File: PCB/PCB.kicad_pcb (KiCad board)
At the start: 2 copper layers, 115 x 77 mm, 153 parts, among them J1 Conn_01x06, J2 Screw_Terminal_01x04, J3 Screw_Terminal_01x08, J4 Conn_02x06_Odd_Even, J5 Conn_01x03, U1 ESP32-S3, U10 TPS22918DBV, U2 PC817, U3 PC817, U4 ADuM1411, U5 ATM90E36A-AU-R, U6 HLK-5M05, U7 B0303S-1WR3, U8 BQ24073RGT, U9 TLV75733PDRV, Y1 ABM8W-16.3840MHZ-4-B1U-T3

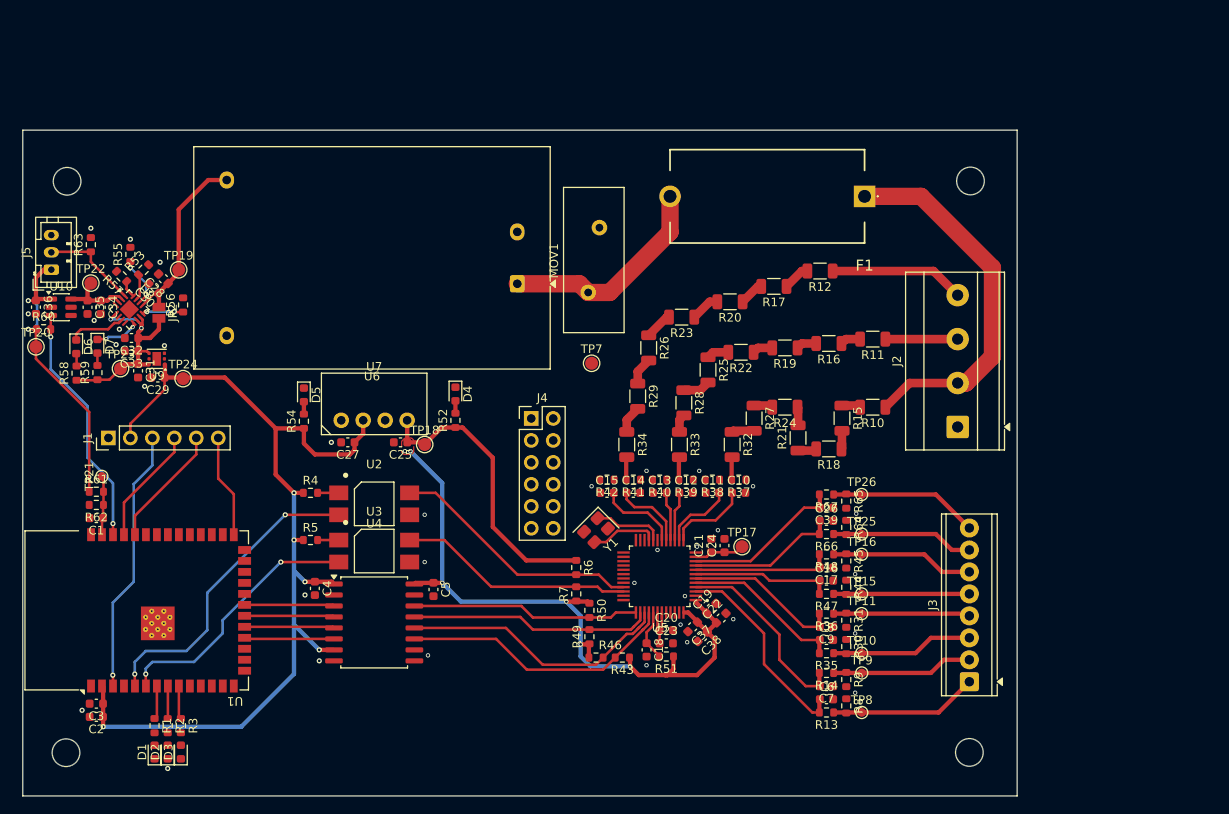
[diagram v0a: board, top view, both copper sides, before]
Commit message: edited the PCB layout
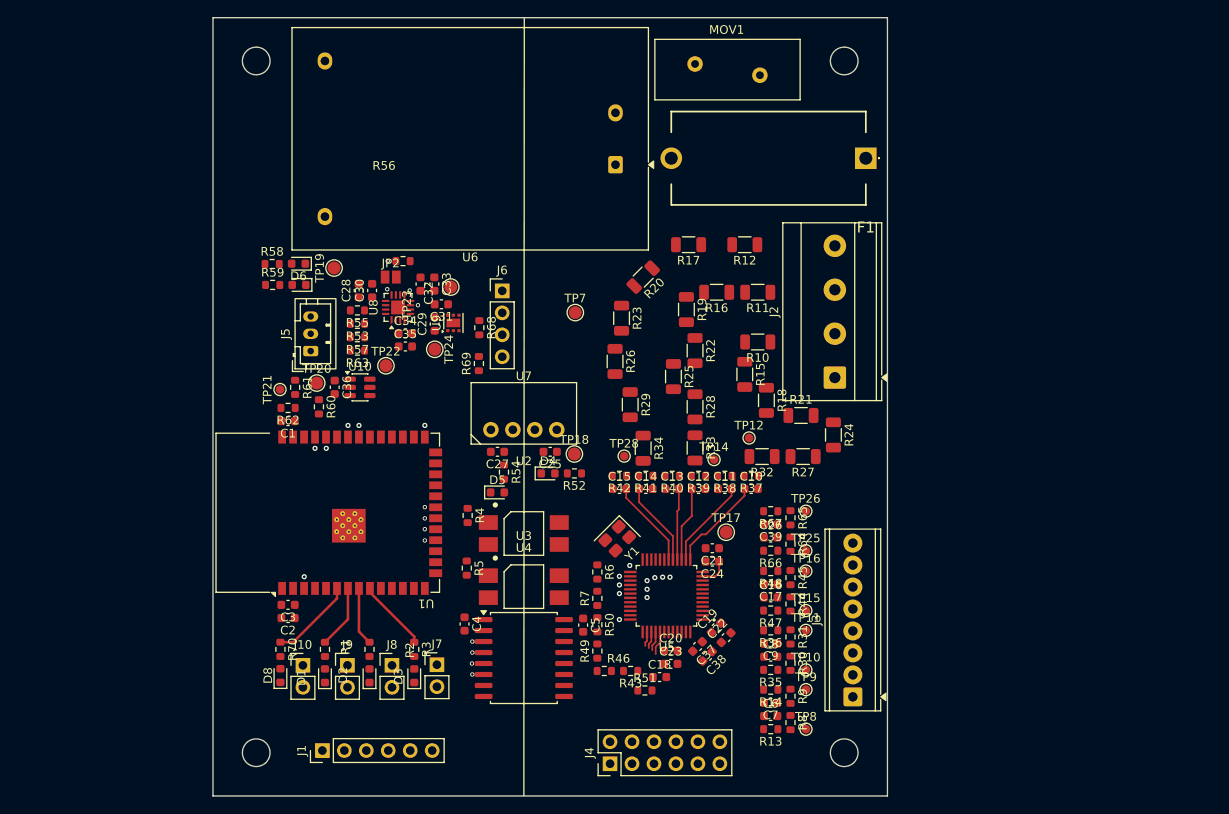
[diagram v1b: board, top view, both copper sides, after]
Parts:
- added D8: LED_L3, LED_SMD:LED_0603_1608Metric, F.Cu at (89.8, 126.1)
- added J10: Conn_01x02, Connector_PinHeader_2.54mm:PinHeader_1x02_P2.54mm_Vertical, F.Cu at (92.4, 124.9)
- added J6: Conn_01x04, Connector_PinHeader_2.54mm:PinHeader_1x04_P2.54mm_Vertical, F.Cu at (115.5, 81.6)
- added J7: Conn_01x02, Connector_PinHeader_2.54mm:PinHeader_1x02_P2.54mm_Vertical, F.Cu at (107.9, 124.8)
- added J8: Conn_01x02, Connector_PinHeader_2.54mm:PinHeader_1x02_P2.54mm_Vertical, F.Cu at (102.7, 124.9)
- added J9: Conn_01x02, Connector_PinHeader_2.54mm:PinHeader_1x02_P2.54mm_Vertical, F.Cu at (97.5, 124.9)
- added R68: 10k, Resistor_SMD:R_0603_1608Metric, F.Cu at (112.8, 85.8)
- added R69: 10k, Resistor_SMD:R_0603_1608Metric, F.Cu at (112.8, 90.0)
- added R70: 1k, Resistor_SMD:R_0603_1608Metric, F.Cu at (89.8, 123.0)
- added TP12: TestPoint, TestPoint:TestPoint_Pad_D1.0mm, F.Cu at (144.0, 98.6)
- added TP14: TestPoint, TestPoint:TestPoint_Pad_D1.0mm, F.Cu at (139.9, 101.1)
- added TP28: TestPoint, TestPoint:TestPoint_Pad_D1.0mm, F.Cu at (129.6, 100.7)
- moved J1 43.8 mm to (94.7, 134.8)
- moved J4 41.0 mm to (127.9, 136.3), turned to 90 degrees
- moved TP23 39.3 mm to (109.5, 81.2), turned to -90 degrees
- moved C35 37.0 mm to (104.3, 88.0), turned to 0 degrees
- moved C31 35.9 mm to (108.4, 83.1), turned to 180 degrees
- moved C33 35.9 mm to (107.6, 80.8), turned to -90 degrees
- moved U10 35.8 mm to (99.0, 92.8)
- moved C36 35.8 mm to (96.1, 92.7)
- moved TP22 35.4 mm to (102.0, 90.2)
- moved C34 35.4 mm to (104.3, 86.5), turned to 0 degrees
- moved U9 34.6 mm to (109.8, 85.3), turned to 90 degrees
- moved C32 34.0 mm to (106.0, 80.8), turned to -90 degrees
- moved R63 33.2 mm to (98.7, 88.5), turned to 180 degrees
- moved R60 33.1 mm to (94.2, 95.0), turned to -90 degrees
- moved TP20 32.7 mm to (94.0, 92.2)
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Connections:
- net /Digital/EN renamed /EN
- net /Digital/IO0 renamed /IO0
- net /Digital/IO14 renamed /IO14
- net /Digital/IO17 renamed /IO17
- net /Digital/IO18 renamed /IO18
- net /Digital/IO21 renamed /IO21
- net /Digital/IO3 renamed /IO3
- net /Digital/IO35 renamed /IO35
- net /Digital/IO36 renamed /IO36
- net /Digital/IO37 renamed /IO37
- net /Digital/IO38 renamed /IO38
- net /Digital/IO39 renamed /IO39
- net /Digital/IO4 renamed /IO4
- net /Digital/IO42 renamed /IO42
- net /Digital/IO46 renamed /IO46
- net /Digital/IO47 renamed /IO47
- net /Digital/IO8 renamed /IO8
- net /Digital/IO9 renamed /IO9
- net /Digital/LED_L1 renamed /LED_L1
- net /Digital/LED_L2 renamed /LED_L2
- net /Digital/LED_L3 renamed /LED_L3
- net /Digital/MCU_CS renamed /MCU_CS
- net /Digital/MCU_MISO renamed /MCU_MISO
- net /Digital/MCU_MOSI renamed /MCU_MOSI
- net /Digital/MCU_SCLK renamed /MCU_SCLK
- net /Digital/RXD0 renamed /RXD0
- net /Digital/TXD0 renamed /TXD0
- net /Digital/USB_D+ renamed /USB_D+
- net /Digital/USB_D- renamed /USB_D-
- net /Energy Metering/I1N renamed /I1N
- net /Energy Metering/I1P renamed /I1P
- net /Energy Metering/I2N renamed /I2N
- net /Energy Metering/I2P renamed /I2P
- net /Energy Metering/I3N renamed /I3N
- net /Energy Metering/I3P renamed /I3P
- net /Energy Metering/I4N renamed /I4N
- net /Energy Metering/I4P renamed /I4P
- net /Energy Metering/OSCI renamed /OSCI
- net /Energy Metering/OSCO renamed /OSCO
- net /Energy Metering/V1N renamed /V1N
- net /Energy Metering/V1P renamed /V1P
- net /Energy Metering/V2N renamed /V2N
- net /Energy Metering/V2P renamed /V2P
- net /Energy Metering/V3N renamed /V3N
- net /Energy Metering/V3P renamed /V3P
- net /Energy Metering/VREF renamed /VREF
- net /Supply/CHG renamed /CHG
- net /Supply/ILIM renamed /ILIM
- net /Supply/ISET renamed /ISET
- net /Supply/PG renamed /PG
- net /Supply/TD renamed /TD
- net /Supply/TMR renamed /TMR
- net /Supply/TS renamed /TS
- J4 pad 1: /Energy Metering/CF4 -> /IRQ0
- J4 pad 10: /Energy Metering/CF2 -> /ZX2
- J4 pad 12: /Energy Metering/CF3 -> /ZX0
- J4 pad 2: /Energy Metering/ZX0 -> /DMA
- J4 pad 3: /Energy Metering/WARN -> /CF2
- J4 pad 4: /Energy Metering/ZX1 -> /CF4
- J4 pad 5: /Energy Metering/IRQ0 -> /IRQ1
- J4 pad 6: /Energy Metering/ZX2 -> /CF1
- J4 pad 7: /Energy Metering/IRQ1 -> /CF3
- J4 pad 8: /Energy Metering/CF1 -> /WARN
- J4 pad 9: /Energy Metering/DMA -> /ZX1
- U1 pad 25: /Digital/IO48 -> /PMC_1
- U1 pad 26: /Digital/IO45 -> /PMC_0
- U1 pad 33: /Digital/IO40 -> /SDA
- U1 pad 34: /Digital/IO41 -> /SCL
- U1 pad 5: /Digital/PMC_0 -> /IO5
- U1 pad 6: /Digital/PMC_1 -> /LED_WIFI
- U2 pad 2: /Digital/PMC_0 -> /PMC_0
- U3 pad 2: /Digital/PMC_1 -> /PMC_1
- U5 pad 22: /Energy Metering/ZX0 -> /ZX0
- U5 pad 23: /Energy Metering/ZX1 -> /ZX1
- U5 pad 24: /Energy Metering/ZX2 -> /ZX2
- U5 pad 25: /Energy Metering/CF1 -> /CF1
- U5 pad 26: /Energy Metering/CF2 -> /CF2
- U5 pad 27: /Energy Metering/CF3 -> /CF3
- U5 pad 28: /Energy Metering/CF4 -> /CF4
- U5 pad 29: /Energy Metering/WARN -> /WARN
- U5 pad 30: /Energy Metering/IRQ0 -> /IRQ0
- U5 pad 31: /Energy Metering/IRQ1 -> /IRQ1
- U5 pad 36: /Energy Metering/DMA -> /DMA
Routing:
- net +3V3PWR: track 114.7 -> 0.00 mm, vias 6 -> 0
- net +3V3: track 112.8 -> 0.00 mm, vias 5 -> 0
- net L1: track 43.3 -> 0.00 mm
- net /Digital/PMC_0: track 36.0 -> 0.00 mm, vias 2 -> 0
- net +VBAT_IN: track 34.6 -> 0.00 mm, vias 2 -> 0
- net /EN: track 30.6 -> 0.00 mm
- net /Digital/PMC_1: track 30.3 -> 0.00 mm, vias 2 -> 0
- net MISO: track 32.3 -> 2.28 mm
- net MOSI: track 31.8 -> 1.99 mm
- net PM0: track 29.3 -> 0.00 mm
- net BAT_SW: track 28.4 -> 0.00 mm, vias 2 -> 0
- net PM1: track 27.2 -> 0.00 mm
- net +VIN: track 26.4 -> 0.00 mm, vias 2 -> 0
- net ~{CS}: track 26.4 -> 0.00 mm
- net SCLK: track 28.1 -> 1.69 mm
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- removed copper zone on F.Cu, net +3V3PWR
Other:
- board size 115 x 77 mm -> 78 x 90 mm

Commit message: PCB routing and adjusts
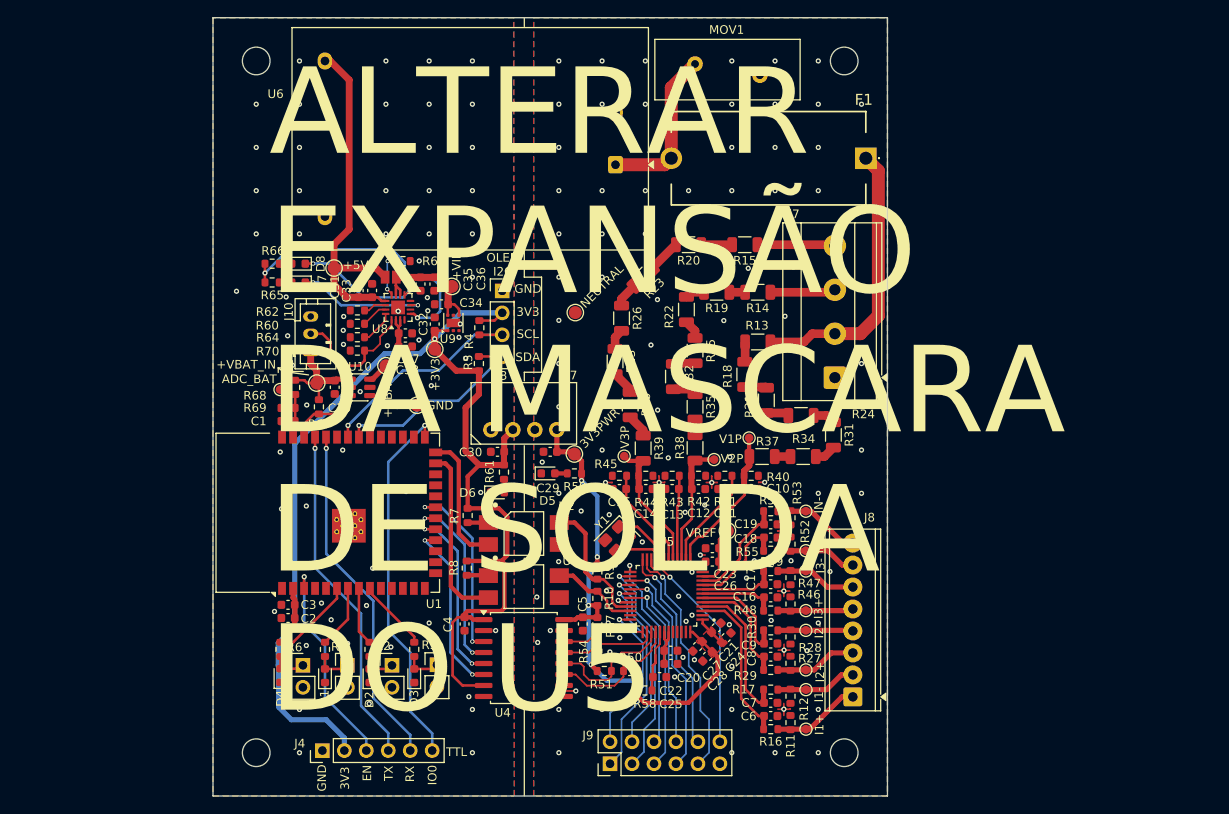
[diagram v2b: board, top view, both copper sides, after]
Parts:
- added TP21: TestPoint, TestPoint:TestPoint_Pad_D1.5mm, F.Cu at (105.6, 94.8)
- moved D8 2.45 mm to (91.9, 78.4)
- moved R66 2.45 mm to (88.8, 78.4)
- moved D7 2.17 mm to (91.9, 80.6)
- moved R65 2.13 mm to (88.8, 80.6)
- moved TP13 0.21 mm to (141.5, 109.3)
- moved TP17 0.16 mm to (109.6, 81.1)
- moved C5 0.13 mm to (124.8, 120.1)
- renumbered C26 to C18, C39 to C19, C18 to C20, C19 to C21, C20 to C22, C21 to C23, C22 to C24, C23 to C25, C24 to C26, C37 to C27, C38 to C28, C25 to C29, C27 to C30, C28 to C31, C29 to C32, C30 to C33, C31 to C34, C32 to C35, C33 to C36, C34 to C37, C35 to C38, C36 to C39, D8 to D4, D4 to D5, D5 to D6, D6 to D7, D7 to D8, J9 to J1, J5 to J10, J8 to J2, J6 to J3, J1 to J4, J7 to J5, J10 to J6, J2 to J7, J3 to J8, J4 to J9, JP2 to JP1, R7 to R10, R8 to R11, R9 to R12, R10 to R13, R11 to R14, R12 to R15, R13 to R16, R14 to R17, R15 to R18, R16 to R19, R17 to R20, R18 to R21, R19 to R22, R20 to R23, R21 to R24, R22 to R25, R23 to R26, R30 to R27, R31 to R28, R35 to R29, R36 to R30, R24 to R31, R25 to R32, R26 to R33, R27 to R34, R28 to R35, R29 to R36, R32 to R37, R33 to R38, R34 to R39, R68 to R4, R37 to R40, R38 to R41, R39 to R42, R40 to R43, R41 to R44, R42 to R45, R44 to R46, R45 to R47, R47 to R48, R48 to R49, R69 to R5, R43 to R50, R46 to R51, R64 to R52, R65 to R53, R49 to R54, R66 to R55, R67 to R56, R50 to R57, R51 to R58, R52 to R59, R70 to R6, R53 to R60, R54 to R61, R55 to R62, R56 to R63, R57 to R64, R58 to R65, R59 to R66, R60 to R67, R61 to R68, R62 to R69, R4 to R7, R63 to R70, R5 to R8, R6 to R9, TP7 to TP1, TP28 to TP10, TP25 to TP11, TP26 to TP12, TP17 to TP13, TP18 to TP14, TP19 to TP15, TP24 to TP16, TP23 to TP17, TP22 to TP18, TP20 to TP19, TP8 to TP2, TP21 to TP20, TP9 to TP3, TP10 to TP4, TP11 to TP5, TP15 to TP6, TP16 to TP7, TP12 to TP8, TP14 to TP9
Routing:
- net +3V3: track 0.00 -> 153.9 mm, vias 0 -> 2
- net +3V3PWR: track 0.00 -> 70.8 mm, vias 0 -> 5
- net +VIN: track 0.00 -> 49.0 mm, vias 0 -> 3
- net /IO0: track 0.00 -> 42.8 mm
- net +5V_EXT: track 0.00 -> 41.2 mm
- net /RXD0: track 0.00 -> 40.3 mm
- net /TXD0: track 0.00 -> 39.8 mm
- net L1: track 0.00 -> 32.6 mm
- net /ZX1: track 0.00 -> 27.6 mm
- net /SCL: track 0.00 -> 26.2 mm
- net /CF2: track 0.00 -> 25.7 mm
- net /CF3: track 0.00 -> 25.5 mm
- net /ZX0: track 0.00 -> 24.9 mm
- net /EN: track 0.00 -> 24.4 mm
- net /ZX2: track 0.00 -> 24.2 mm
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- added copper zone on F.Cu, net +3V3PWR
- added copper zone on B.Cu, net GND
- added copper zone on F.Cu, net GND
- added copper zone on B.Cu, net N
- added copper zone on F.Cu, net N
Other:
- board text added: "+3V3"
- board text added: "+5V"
- board text added: "+VBAT"
- board text added: "+VBAT_IN"
- board text added: "+VIN"
- board text added: "3V3"
- board text added: "3V3PWR"
- board text added: "ADC_BAT"
- board text added: "ALTERAR EXPANSÃO DA MASCARA DE SOLDA DO U5"
- board text added: "EN"
- board text added: "GND"
- board text added: "I1+"
- board text added: "I1-"
- board text added: "I2+"
- board text added: "I2-"
- board text added: "I3+"
- board text added: "I3-"
- board text added: "IN+"
- board text added: "IN-"
- board text added: "IO0"
- board text added: "NEUTRAL"
- board text added: "OLED I2C"
- board text added: "RX"
- board text added: "SCL"
- board text added: "SDA"
- board text added: "TTL"
- board text added: "TX"
- board text added: "V1P"
- board text added: "V2P"
- board text added: "V3P"
- board text added: "VREF"
